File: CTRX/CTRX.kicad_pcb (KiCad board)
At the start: 2 copper layers, 45 x 19 mm, 33 parts, among them J1 CON-SMA-EDGE-S, J3 Conn_02x05_Odd_Even, J4 USB-AM-S-X-X-TH, U1 nRF52820-QDxx, U2 NRF21540-QDAA-R7, U3 USBLC6-2SC6, U4 ME6211C33M5, Y1 32MHz

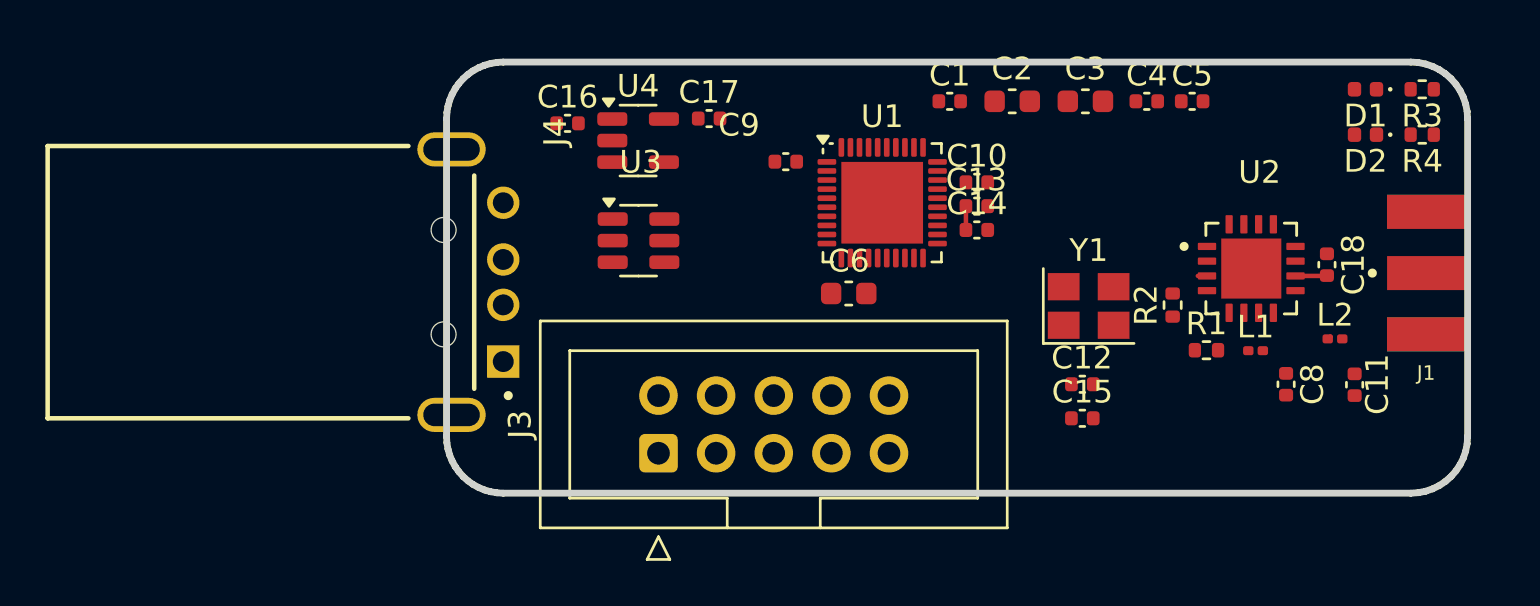
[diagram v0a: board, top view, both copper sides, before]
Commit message: CTRX updated
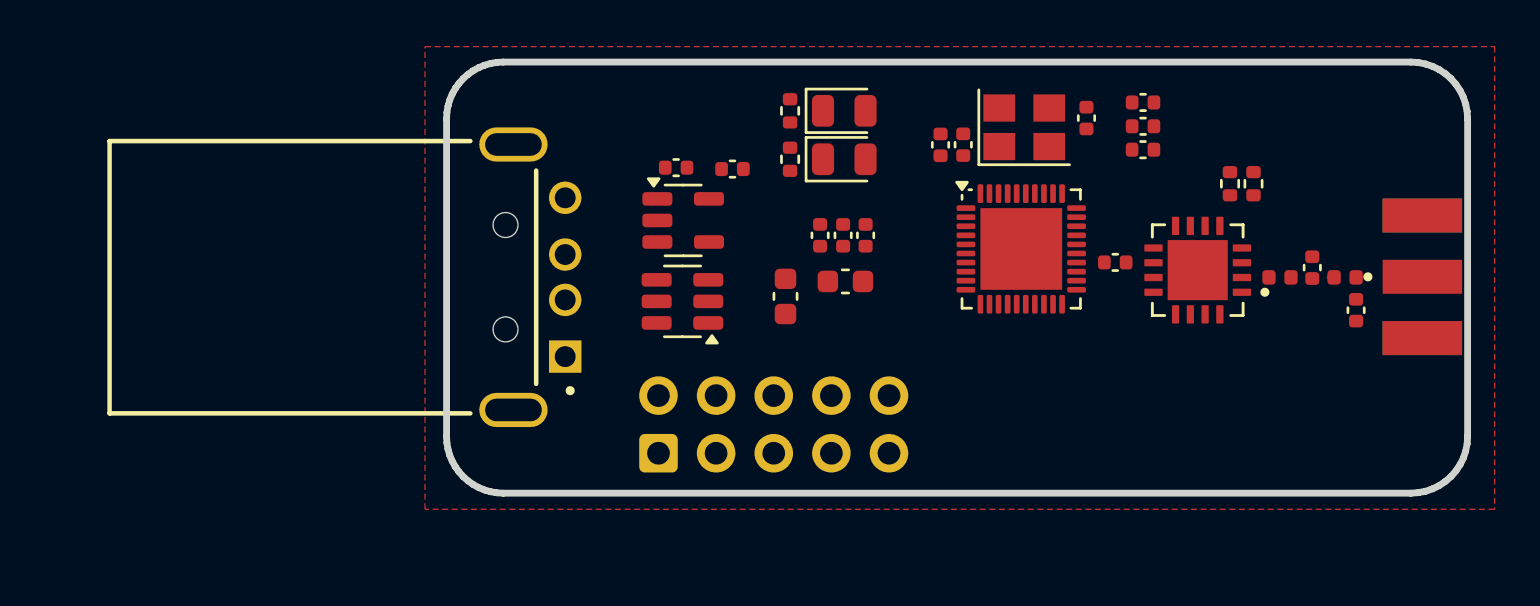
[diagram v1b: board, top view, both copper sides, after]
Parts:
- removed C2: 4.7uF, Capacitor_SMD:C_0603_1608Metric
- D1, D2: footprint LED_SMD:LED_0402_1005Metric -> LED_SMD:LED_0805_2012Metric
- L1, L2: footprint Inductor_SMD:L_0201_0603Metric -> Inductor_SMD:L_0402_1005Metric
- moved R3 28.0 mm to (129.6, 83.1), turned to -90 degrees
- moved R4 27.9 mm to (129.6, 80.9), turned to 90 degrees
- moved D1 23.2 mm to (132.0, 83.1), turned to 0 degrees
- moved D2 23.0 mm to (132.0, 80.9), turned to 0 degrees
- moved C3 15.8 mm to (129.4, 89.1), turned to 90 degrees
- moved C4 15.6 mm to (131.0, 86.4), turned to -90 degrees
- moved C5 15.6 mm to (133.0, 86.4), turned to -90 degrees
- moved C15 13.2 mm to (142.7, 81.3), turned to 90 degrees
- moved C12 11.8 mm to (137.3, 82.4), turned to -90 degrees
- moved C18 9.33 mm to (144.0, 87.6), turned to 0 degrees
- moved C13 8.63 mm to (145.2, 80.6)
- moved C14 8.63 mm to (145.2, 81.6)
- moved Y1 8.37 mm to (140.0, 81.7)
- moved C1 7.55 mm to (132.0, 86.4), turned to 90 degrees
- moved C10 7.46 mm to (145.2, 82.7)
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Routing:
- net Net-(U2-TRX): track 1.39 -> 0.00 mm
- net DEC4: track 1.05 -> 0.00 mm
- net Net-(C11-Pad1): track 1.00 -> 0.00 mm
- added copper zone on F.Cu, net GND
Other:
- copper layers 2 -> 4
